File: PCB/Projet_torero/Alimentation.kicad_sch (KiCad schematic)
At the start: 20 parts, among them IC501 MP1475SGJ-P, J501 Conn_01x02, U501 BU33SD5WG-TR

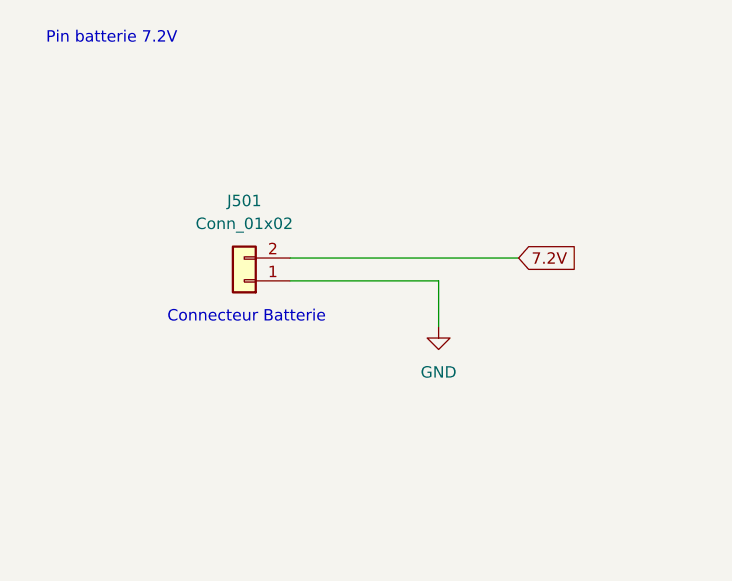
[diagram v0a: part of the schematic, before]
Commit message: Mis à jour des composants
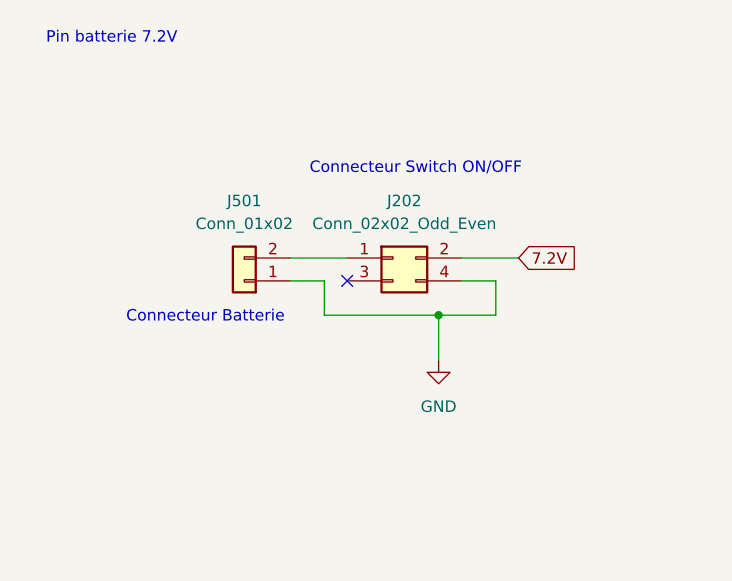
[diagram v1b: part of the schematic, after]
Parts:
- added J202: Conn_02x02_Odd_Even, symbol Connector_Generic:Conn_02x02_Odd_Even
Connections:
- net 7.2V: now also J202.2 (Pin_2); no longer J501.2 (Pin_2)
- net GND: now also J202.4 (Pin_4)
- new net: J202.1 (Pin_1), J501.2 (Pin_2)
- no-connect marks 0 -> 1
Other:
- note added: "Connecteur Switch ON/OFF"
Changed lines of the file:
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@@
 		(color 0 0 0 0)
 	)
+	(junction
+		(at 57.15 44.45)
+		(diameter 0)
+		(color 0 0 0 0)
+	)
+	(no_connect
+		(at 46.99 40.64)
+	)
 	(polyline
 		(pts
@@
 	(wire
 		(pts
+			(xy 63.5 40.64) (xy 63.5 44.45)
+		)
+		(stroke
+			(width 0)
+			(type default)
+		)
+	)
+	(wire
+		(pts
 			(xy 203.2 120.65) (xy 203.2 127)
 		)
@@
 	(wire
 		(pts
+			(xy 63.5 44.45) (xy 57.15 44.45)
+		)
+		(stroke
+			(width 0)
+			(type default)
+		)
+	)
+	(wire
+		(pts
 			(xy 227.33 138.43) (xy 227.33 139.7)
 		)
@@
 	(wire
 		(pts
+			(xy 44.45 40.64) (xy 44.45 44.45)
+		)
+		(stroke
+			(width 0)
+			(type default)
+		)
+	)
+	(wire
+		(pts
 			(xy 71.12 152.4) (xy 64.77 152.4)
 		)
@@
 	(wire
 		(pts
-			(xy 57.15 40.64) (xy 57.15 45.72)
-		)
-		(stroke
-			(width 0)
-			(type default)
-		)
-	)
-	(wire
-		(pts
-			(xy 57.15 40.64) (xy 40.64 40.64)
-		)
-		(stroke
-			(width 0)
-			(type default)
-		)
-	)
-	(wire
-		(pts
 			(xy 127 156.21) (xy 127 161.29)
 		)
@@
 	(wire
 		(pts
+			(xy 59.69 40.64) (xy 63.5 40.64)
+		)
+		(stroke
+			(width 0)
+			(type default)
+		)
+	)
+	(wire
+		(pts
+			(xy 59.69 38.1) (xy 66.04 38.1)
+		)
+		(stroke
+			(width 0)
+			(type default)
+		)
+	)
+	(wire
+		(pts
 			(xy 115.57 153.67) (xy 115.57 156.21)
 		)
@@
 	(wire
 		(pts
+			(xy 40.64 38.1) (xy 46.99 38.1)
+		)
+		(stroke
+			(width 0)
+			(type default)
+		)
+	)
+	(wire
+		(pts
 			(xy 62.23 138.43) (xy 71.12 138.43)
 		)
@@
 	(wire
 		(pts
-			(xy 40.64 38.1) (xy 66.04 38.1)
-		)
-		(stroke
-			(width 0)
-			(type default)
-		)
-	)
-	(wire
-		(pts
 			(xy 128.27 35.56) (xy 128.27 30.48)
 		)
@@
 	(wire
 		(pts
+			(xy 44.45 44.45) (xy 57.15 44.45)
+		)
+		(stroke
+			(width 0)
+			(type default)
+		)
+	)
+	(wire
+		(pts
 			(xy 71.12 147.32) (xy 71.12 152.4)
+		)
+		(stroke
+			(width 0)
+			(type default)
+		)
+	)
+	(wire
+		(pts
+			(xy 44.45 40.64) (xy 40.64 40.64)
+		)
+		(stroke
+			(width 0)
+			(type default)
+		)
+	)
+	(wire
+		(pts
+			(xy 57.15 44.45) (xy 57.15 49.53)
 		)
 		(stroke
@@
 		)
 	)
+	(text "Connecteur Switch ON/OFF"
+		(exclude_from_sim no)
+		(at 54.61 28.194 0)
+		(effects
+			(font
+				(size 1.27 1.27)
+			)
+		)
+	)
 	(text "Régulateur tension 5V"
 		(exclude_from_sim no)
@@
 	(text "Connecteur Batterie"
 		(exclude_from_sim no)
-		(at 35.814 44.704 0)
+		(at 31.242 44.704 0)
 		(effects
 			(font
@@
 	)
 	(symbol
+		(lib_id "Connector_Generic:Conn_02x02_Odd_Even")
+		(at 52.07 38.1 0)
+		(unit 1)
+		(exclude_from_sim no)
+		(in_bom yes)
+		(on_board yes)
+		(dnp no)
+		(fields_autoplaced yes)
+		(property "Reference" "J202"
+			(at 53.34 31.75 0)
+			(effects
+				(font
+					(size 1.27 1.27)
+				)
+			)
+		)
+		(property "Value" "Conn_02x02_Odd_Even"
+			(at 53.34 34.29 0)
+			(effects
+				(font
+					(size 1.27 1.27)
+				)
+			)
+		)
+		(property "Footprint" ""
+			(at 52.07 38.1 0)
+			(effects
+				(font
+					(size 1.27 1.27)
+				)
+				(hide yes)
+			)
+		)
+		(property "Datasheet" "~"
+			(at 52.07 38.1 0)
+			(effects
+				(font
+					(size 1.27 1.27)
+				)
+				(hide yes)
+			)
+		)
+		(property "Description" "Generic connector, double row, 02x02, odd/even pin numbering scheme (row 1 odd numbers, row 2 even numbers), script generated (kicad-library-utils/schlib/autogen/connector/)"
+			(at 52.07 38.1 0)
+			(effects
+				(font
+					(size 1.27 1.27)
+				)
+				(hide yes)
+			)
+		)
+		(pin "3"
+		)
+		(pin "4"
+		)
+		(pin "2"
+		)
+		(pin "1"
+		)
+		(instances
+			(project ""
+				(path "/04e1eb47-a2c4-462b-bef7-377d9515a2c0/b3b2826c-2e3c-42fe-bcd6-22fcd6249c25"
+					(reference "J202")
+					(unit 1)
+				)
+			)
+		)
+	)
+	(symbol
 		(lib_id "power:GND")
-		(at 57.15 45.72 0)
+		(at 57.15 49.53 0)
 		(unit 1)
 		(exclude_from_sim no)
@@
 		(fields_autoplaced yes)
 		(property "Reference" "#PWR0503"
-			(at 57.15 52.07 0)
+			(at 57.15 55.88 0)
 			(effects
 				(font
@@
 		)
 		(property "Value" "GND"
-			(at 57.15 50.8 0)
+			(at 57.15 54.61 0)
 			(effects
 				(font
@@
 		)
 		(property "Footprint" ""
-			(at 57.15 45.72 0)
+			(at 57.15 49.53 0)
 			(effects
 				(font
@@
 		)
 		(property "Datasheet" ""
-			(at 57.15 45.72 0)
+			(at 57.15 49.53 0)
 			(effects
 				(font
@@
 		)
 		(property "Description" "Power symbol creates a global label with name \"GND\" , ground"
-			(at 57.15 45.72 0)
-			(effects
-				(font
+			(at 57.15 49.53 0)
+			(effects
+				(font
